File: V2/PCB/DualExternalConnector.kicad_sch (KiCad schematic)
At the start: 4 parts, among them J1003 Conn_02x04_Counter_Clockwise, J103 RJ45, J105 DA15_Plug

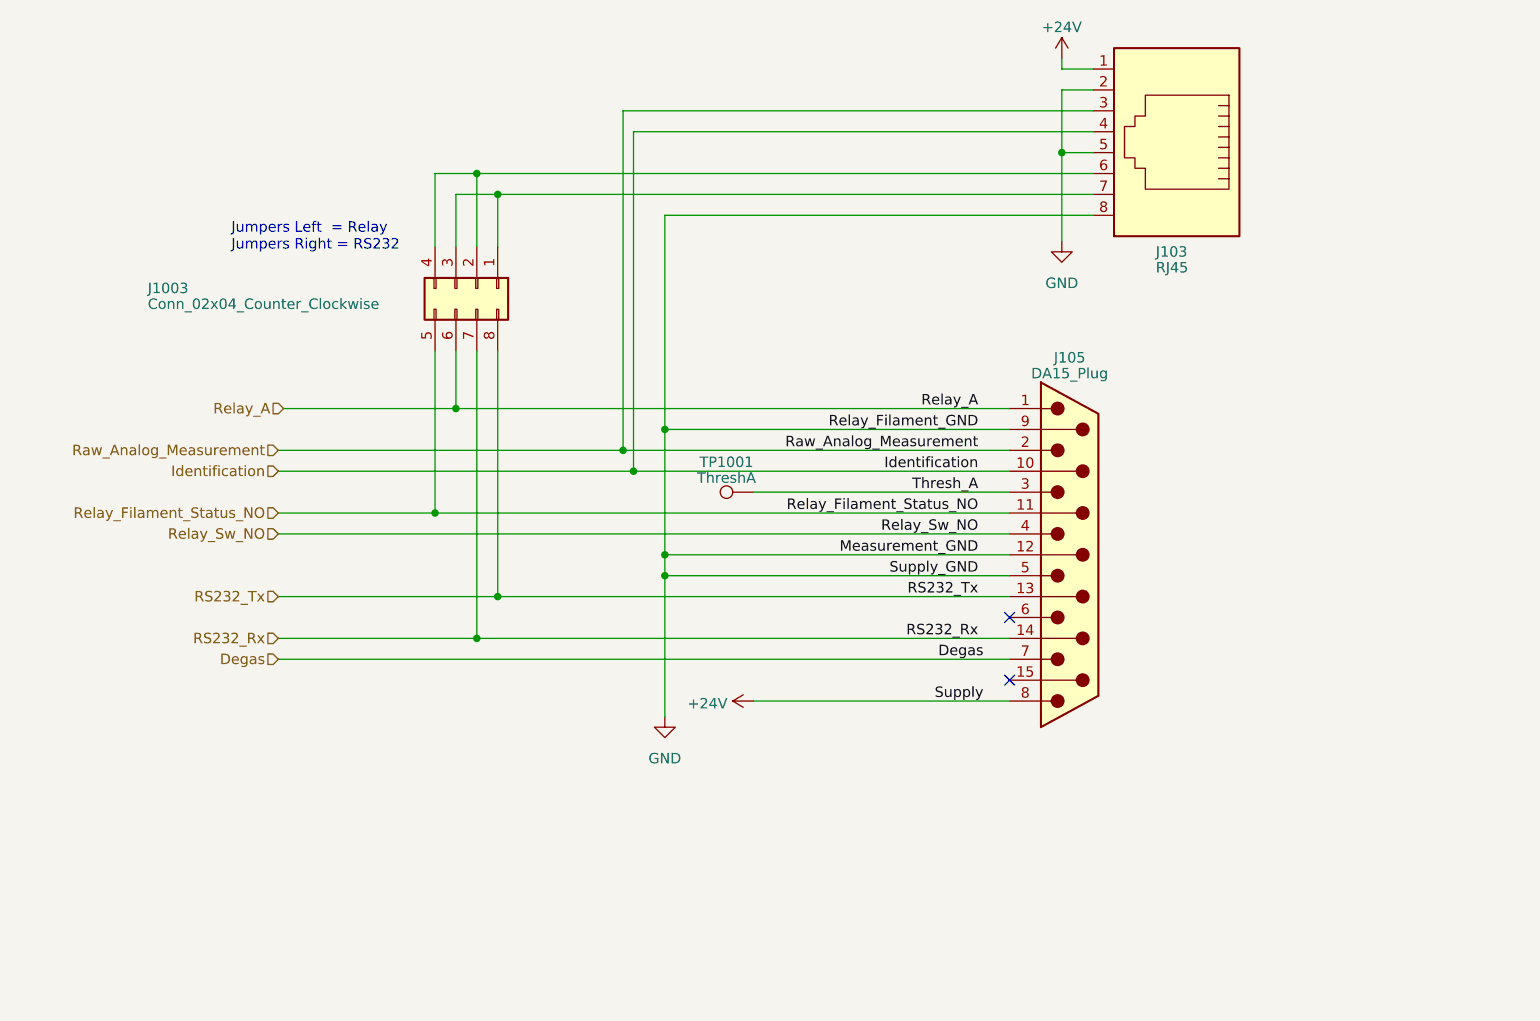
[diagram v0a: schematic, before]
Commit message: Schematic "Finished"
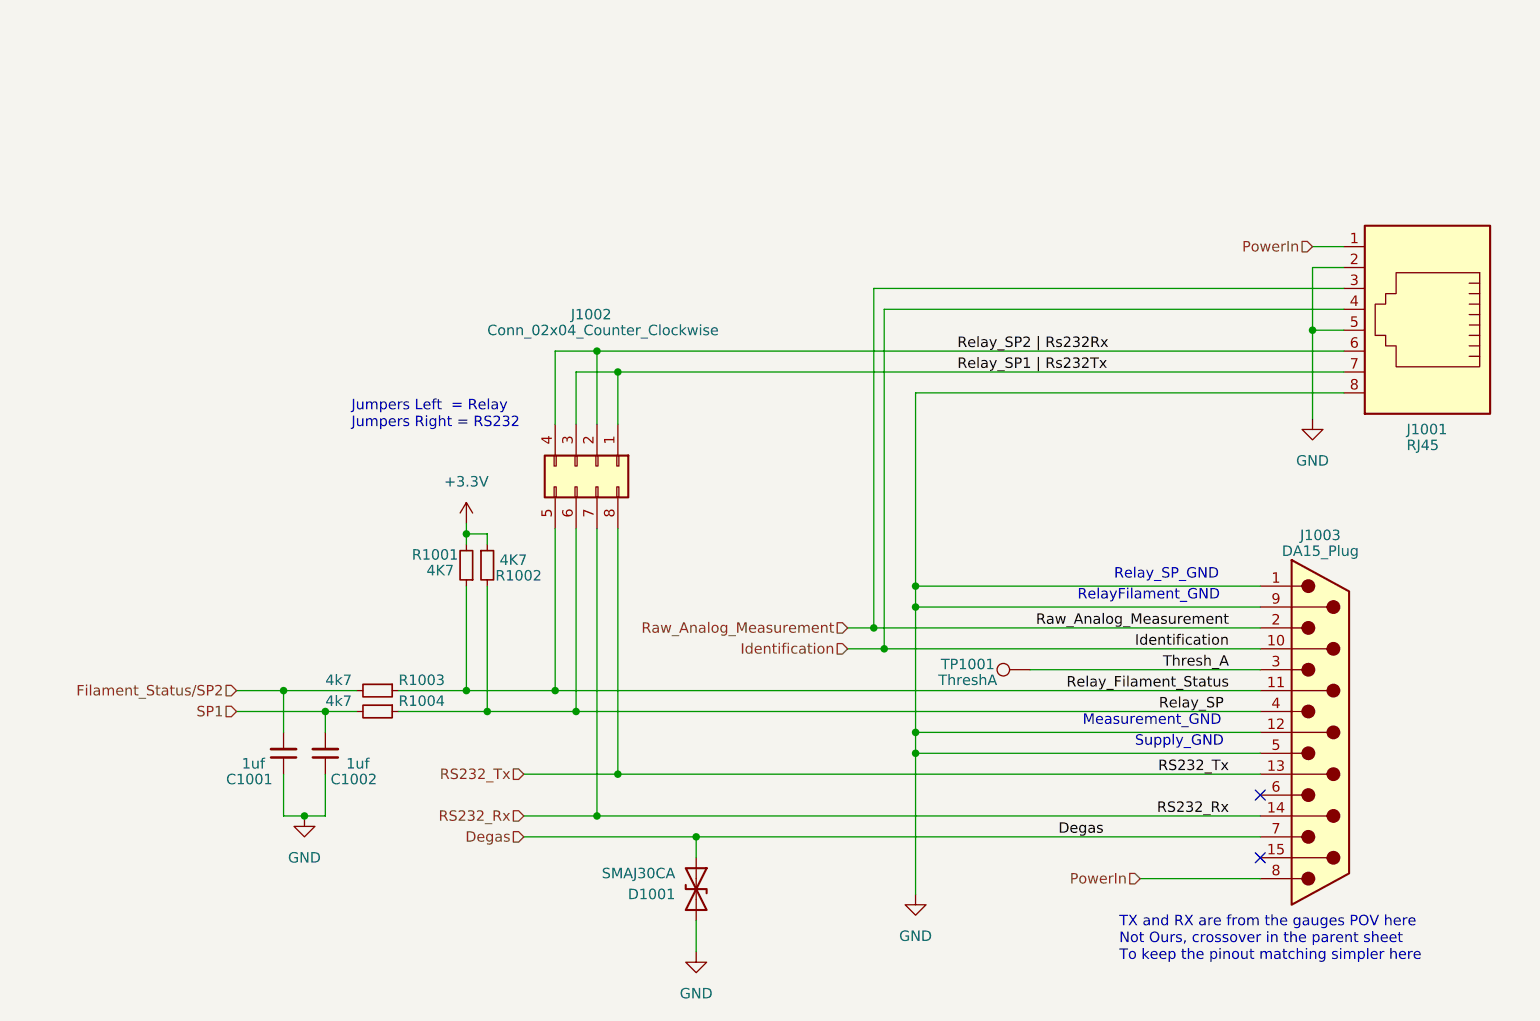
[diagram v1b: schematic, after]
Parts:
- added C1001, C1002: 1uf, Capacitor_SMD:C_0805_2012Metric, symbol PGD-Library:C_Small
- added D1001: SMAJ30CA, Diode_SMD:D_SMA, symbol PGD-Library:D_TVS
- added R1001, R1002: 4K7, Resistor_SMD:R_0805_2012Metric, symbol PGD-Library:R_Small
- added R1003, R1004: 4k7, Resistor_SMD:R_0402_1005Metric, symbol PGD-Library:R_Small
- J1002: renamed from J1003; footprint (none) -> Connector_PinHeader_2.54mm:PinHeader_2x04_P2.54mm_Vertical
- J1003: renamed from J105; footprint Connector_Dsub:DSUB-15_Male_Horizontal_P2.77x2.84mm_EdgePinOffset4.94mm_Housed_MountingHolesOffset7.48mm -> easyeda2kicad2:DSUB-TH_Z-SUBDRBM602A002; JLC Part (none) -> Extended Part; LCSC Part (none) -> C235810; Mfg Part (none) -> DSUB-TH_Z-SUBDRBM602A002
- TP1001: footprint (none) -> TestPoint:TestPoint_Pad_2.0x2.0mm
- renumbered J103 to J1001
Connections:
- net Relay_Sw_NO is gone; now on net Relay_SP: J1003.4
- net Degas: now also D1001.1 (A1)
- net GND: now also J1003.1, C1001.1, C1002.1, D1001.2 (A2)
- net Relay_SP2 | Rs232Rx: now reaches J1001.6, J1002.2 (Pin_2), J1002.4 (Pin_4)
- net Relay_SP1 | Rs232Tx: now reaches J1001.7, J1002.1 (Pin_1), J1002.3 (Pin_3)
- net +24V renamed PowerIn
- net Relay_A renamed Relay_SP
- net Relay_SP: now also R1002.2, R1004.1; no longer J1003.1
- net Relay_Filament_Status_NO renamed Relay_Filament_Status
- net Relay_Filament_Status: now also R1001.1, R1003.1
- new net +3.3V: R1001.2, R1002.1
- new net Filament_Status/SP2: C1001.2, R1003.2
- new net SP1: C1002.2, R1004.2
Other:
- note added: "Measurement_GND"
- note added: "RelayFilament_GND"
- note added: "Relay_SP_GND"
- note added: "Supply_GND"
- note added: "TX and RX are from the gauges POV here Not Ours, crossover in the parent sheet To keep the pinout matching simpler here"
- moved on the sheet: J1001, J1002, J1003, TP1001
